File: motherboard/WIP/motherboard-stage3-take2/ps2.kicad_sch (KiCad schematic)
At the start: 24 parts, among them U29 74HCT32, U30 74HCT14, U31 74HCT595, U32 74HCT595, U33 74HCT574, U34 74HCT595, U35 74HCT595, U36 74ALS576, U9 74HCT14

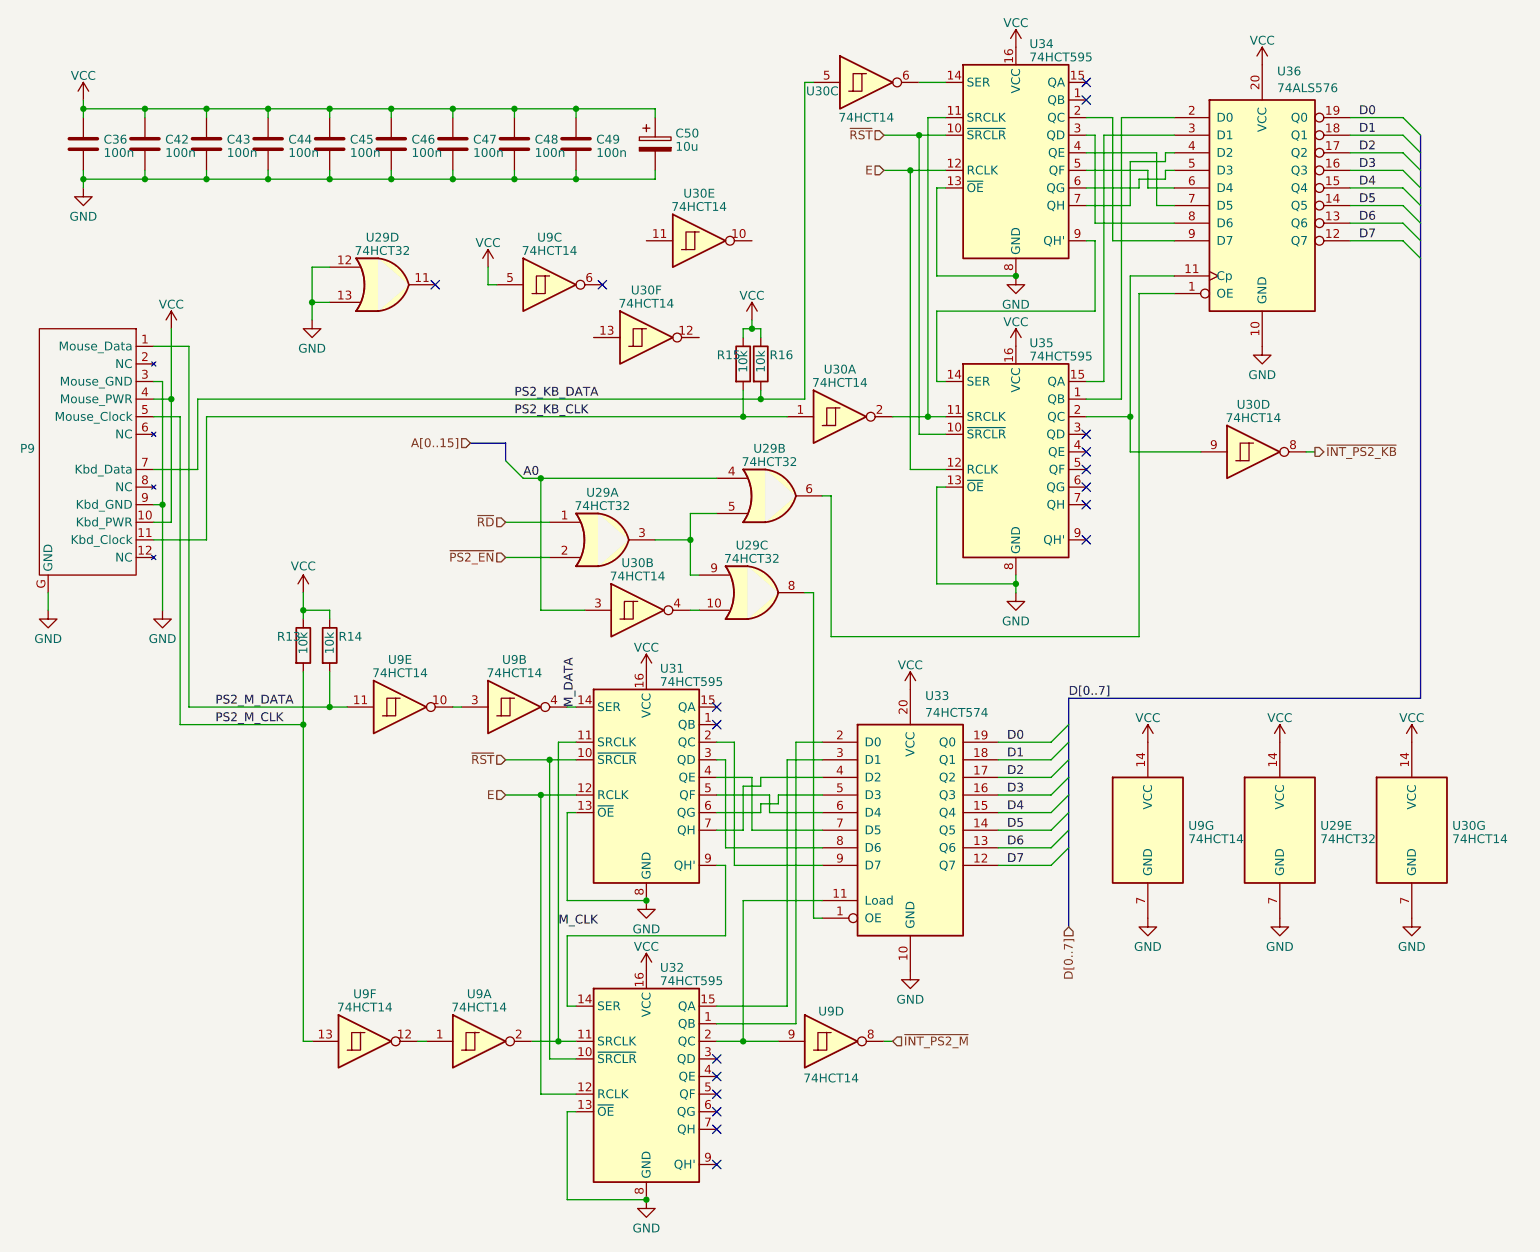
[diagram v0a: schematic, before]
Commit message: Added new ps handling in stage3-rev1
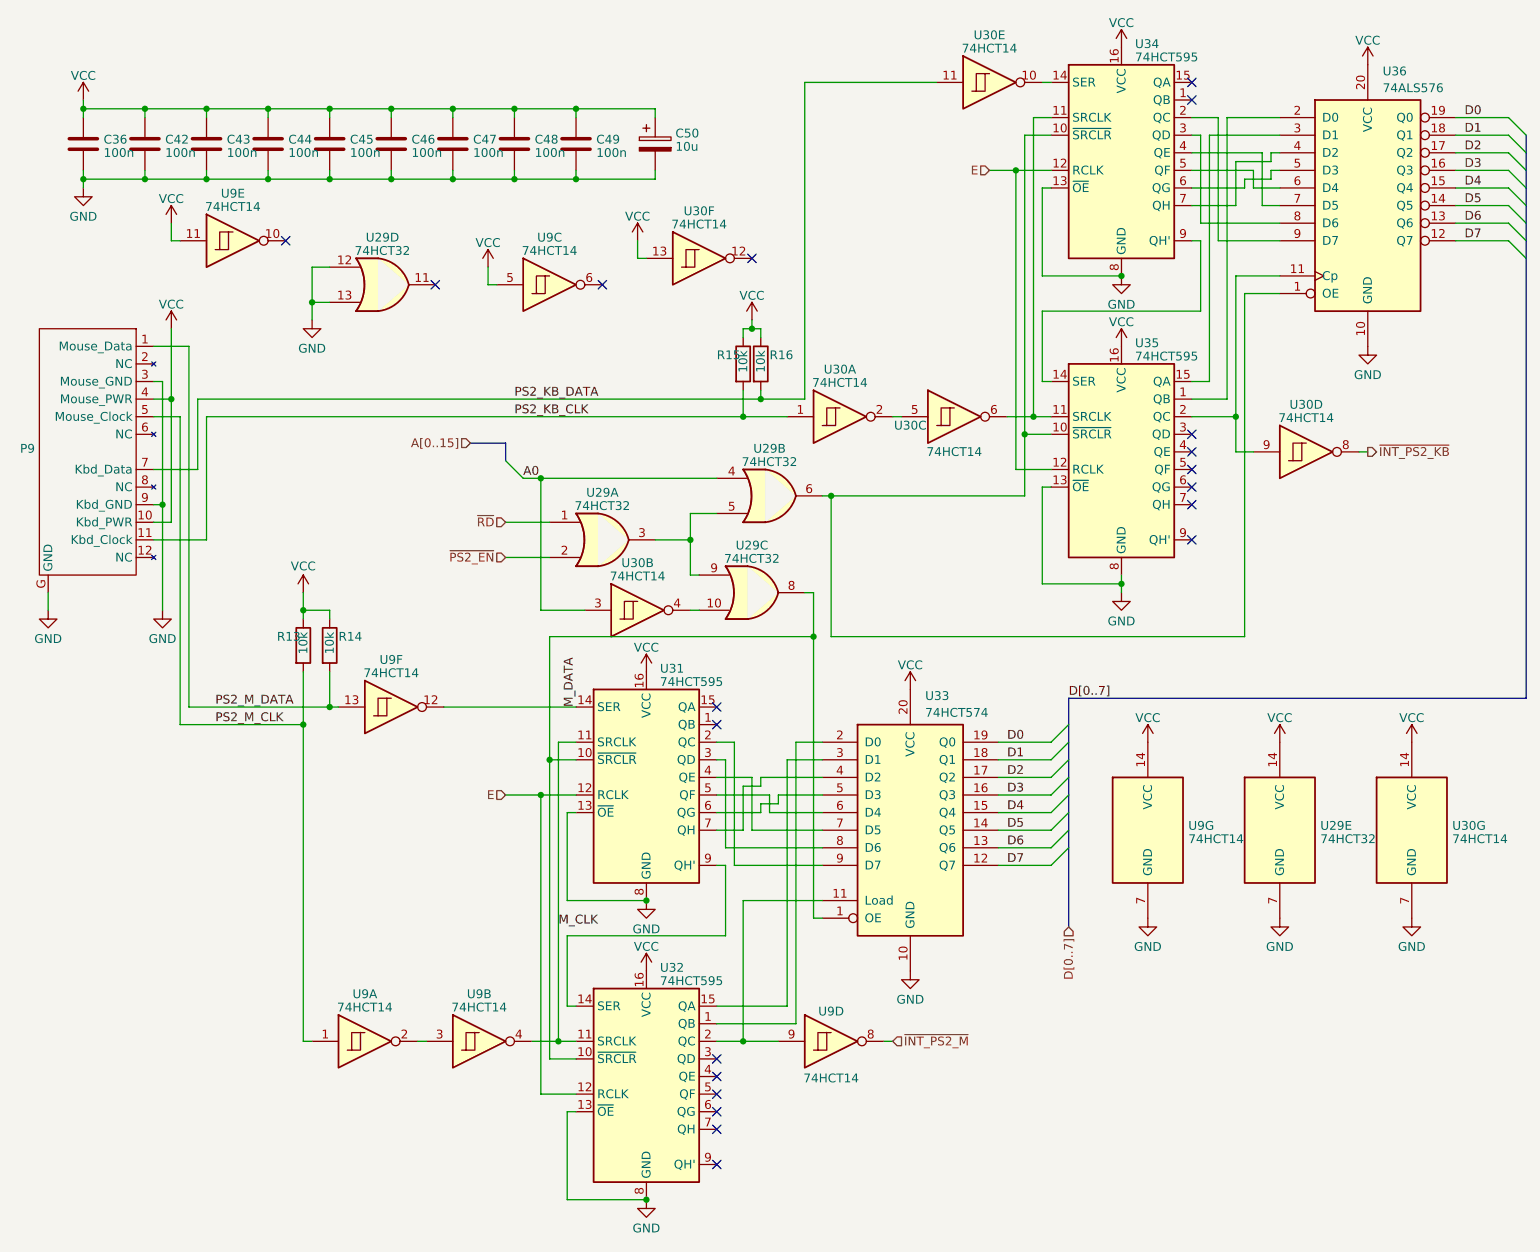
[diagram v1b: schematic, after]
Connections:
- net M_CLK: now also U9.4; no longer U9.2
- net M_DATA: now also U9.12; no longer U9.4
- net PS2_KB_DATA: now also U30.11; no longer U30.5
- net PS2_M_CLK: now also U9.1; no longer U9.13
- net PS2_M_DATA: now also U9.13; no longer U9.11
- net VCC: now also U30.13, U9.11
- net at U29.8, U33.1 (OE): now also U31.10 (~{SRCLR}), U32.10 (~{SRCLR})
- net at U29.6, U36.1 (OE): now also U34.10 (~{SRCLR}), U35.10 (~{SRCLR})
- net at U30.10: now also U34.14 (SER)
- net at U9.3: now also U9.2; no longer U9.10
- net at U34.11 (SRCLK), U35.11 (SRCLK): now also U30.6; no longer U30.2
- removed net ~{RST}: U31.10 (~{SRCLR}), U32.10 (~{SRCLR}), U34.10 (~{SRCLR}), U35.10 (~{SRCLR})
- new net: U30.2, U30.5
- no-connect marks 18 -> 20
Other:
- moved on the sheet: U30C, U30D, U30E, U30F, U34, U35, U36, U9A, U9B, U9E, U9F
